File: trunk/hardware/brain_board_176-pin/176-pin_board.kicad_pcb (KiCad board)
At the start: 4 copper layers, 61.8 x 73.2 mm, 77 parts, among them J1 MINI-USB-5P-3400020P1, P1 CONN_25X2, P10 CONN_2X2, P11 CONN_4X2, P12 CONN_4X2, P13 CONN_8X2, P2 CONN_25X2, P3 CONN_2, P4 CONN_6, P5 CONN_1, P6 CONN_2X2, P7 CONN_4X2, P8 CONN_4X2, P9 CONN_4X2, SW1 SW_PUSH, U1 STM32F407IGT6, U2 NUF2101MT1G, U3 LM2937, X1 CRYSTAL, X2 CRYSTAL

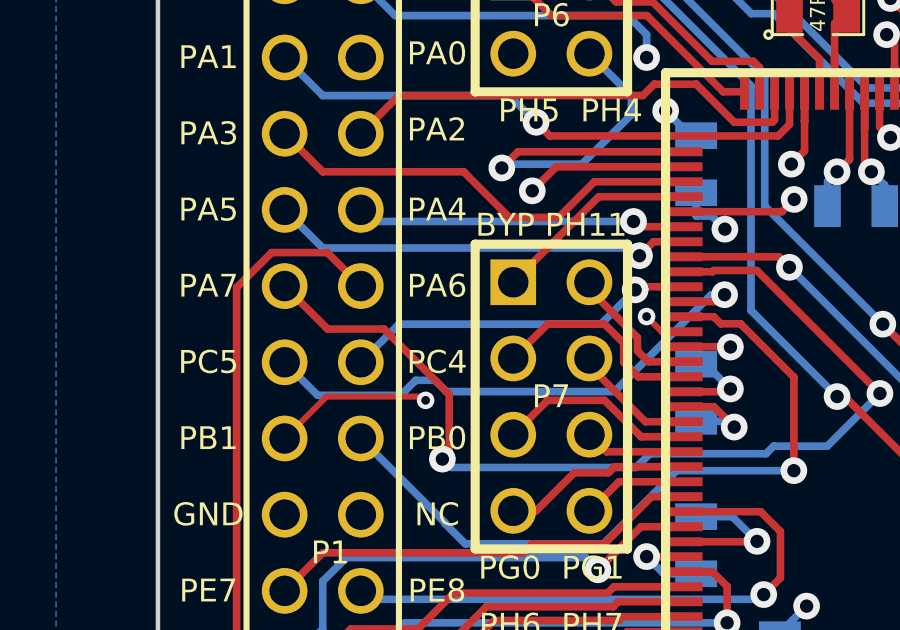
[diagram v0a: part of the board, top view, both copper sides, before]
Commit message: progress
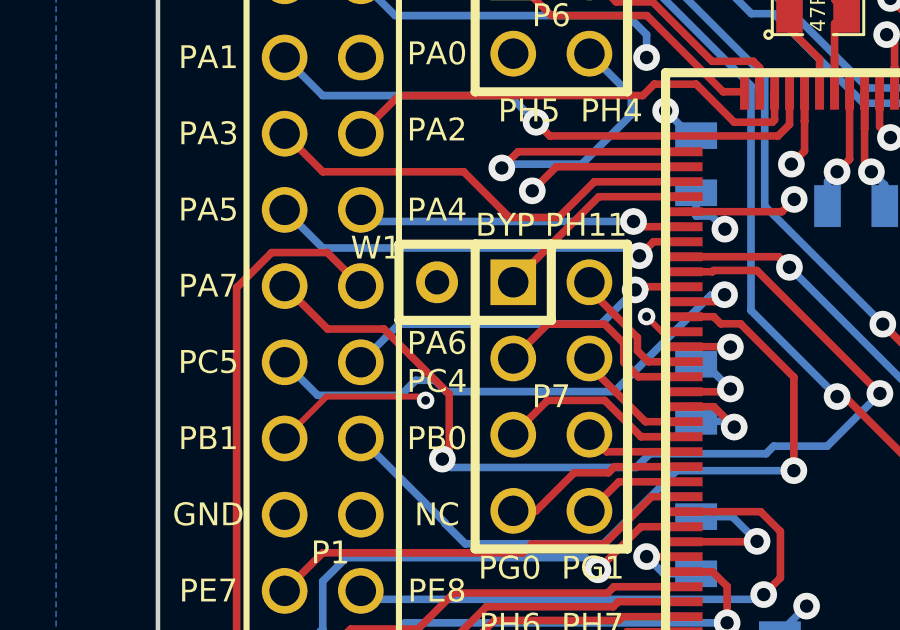
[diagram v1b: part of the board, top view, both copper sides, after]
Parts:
- added W1: TEST, SIL-2, F.Cu at (97.8, 113.7)
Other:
- net class Default: clearance 0.2032 -> 0.1778
- rule trace_clearance: 0.2032 -> 0.1778
